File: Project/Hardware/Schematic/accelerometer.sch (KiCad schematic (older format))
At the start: 2 parts, among them U3 lis3dh_board

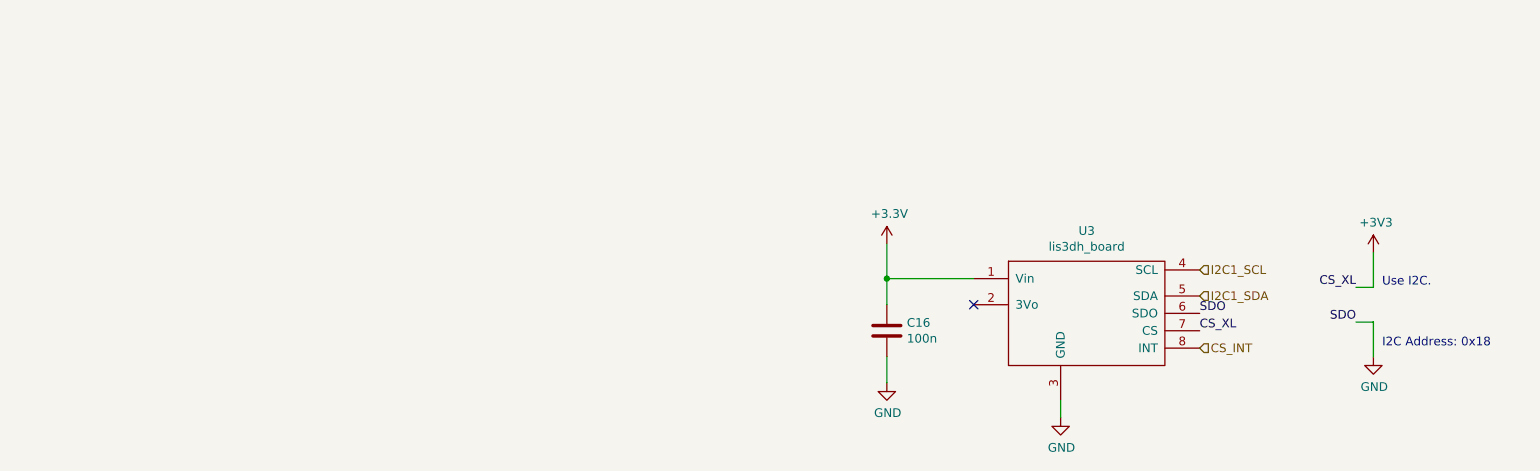
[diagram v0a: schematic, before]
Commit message: Intermediate...
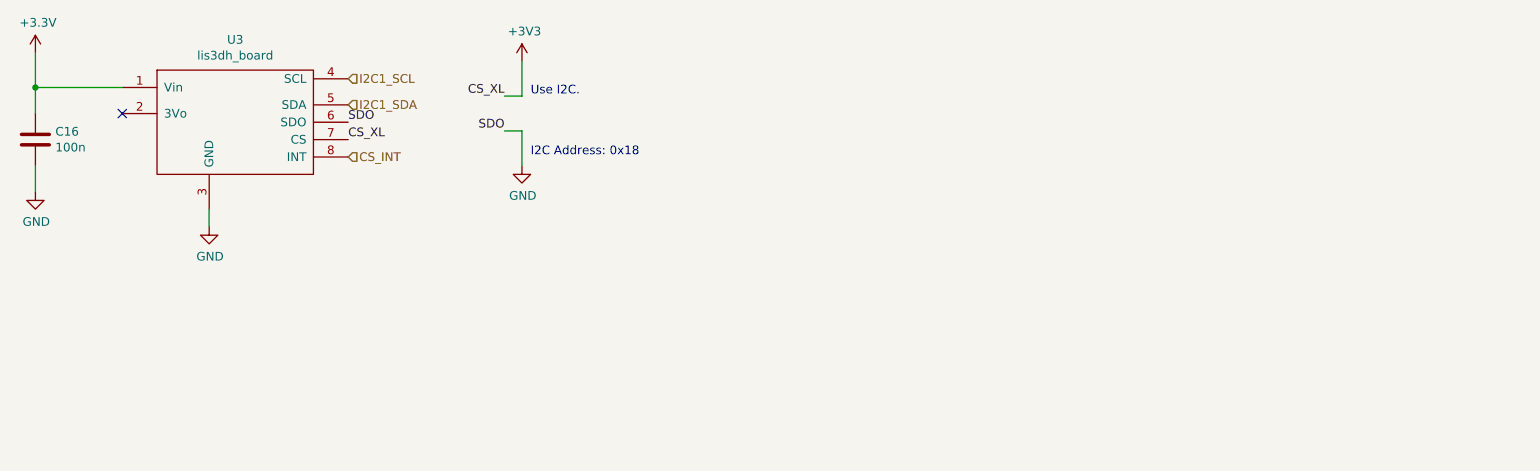
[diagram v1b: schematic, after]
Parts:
- C16: footprint (none) -> Capacitor_SMD:C_0805_2012Metric_Pad1.15x1.40mm_HandSolder
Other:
- moved on the sheet: C16, U3
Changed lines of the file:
@@
 EELAYER 26 0
 EELAYER END
-$Descr A4 11693 8268
+$Descr User 5512 5512
 encoding utf-8
 Sheet 2 7
 Title ""
-Date ""
-Rev ""
-Comp ""
+Date "2019-02-12"
+Rev "1"
+Comp "PASC"
 Comment1 ""
 Comment2 ""
@@
 L power:+3.3V #PWR0120
 U 1 1 5C5AB0A3
-P 6200 2950
-F 0 "#PWR0120" H 6200 2800 50  0001 C CNN
-F 1 "+3.3V" H 6215 3123 50  0000 C CNN
-F 2 "" H 6200 2950 50  0001 C CNN
-F 3 "" H 6200 2950 50  0001 C CNN
-	1    6200 2950
+P 1300 1850
+F 0 "#PWR0120" H 1300 1700 50  0001 C CNN
+F 1 "+3.3V" H 1315 2023 50  0000 C CNN
+F 2 "" H 1300 1850 50  0001 C CNN
+F 3 "" H 1300 1850 50  0001 C CNN
+	1    1300 1850
 	1    0    0    -1
 $EndComp
 Wire Wire Line
-	6200 2950 6200 3150
+	1300 1850 1300 2050
 Wire Wire Line
-	6700 3150 6200 3150
+	1800 2050 1300 2050
 $Comp
 L power:GND #PWR0121
 U 1 1 5C59F3FC
-P 7200 3950
-F 0 "#PWR0121" H 7200 3700 50  0001 C CNN
-F 1 "GND" H 7205 3777 50  0000 C CNN
-F 2 "" H 7200 3950 50  0001 C CNN
-F 3 "" H 7200 3950 50  0001 C CNN
-	1    7200 3950
+P 2300 2850
+F 0 "#PWR0121" H 2300 2600 50  0001 C CNN
+F 1 "GND" H 2305 2677 50  0000 C CNN
+F 2 "" H 2300 2850 50  0001 C CNN
+F 3 "" H 2300 2850 50  0001 C CNN
+	1    2300 2850
 	1    0    0    -1
 $EndComp
 Wire Wire Line
-	7200 3850 7200 3950
+	2300 2750 2300 2850
 $Comp
 L power:GND #PWR0122
 U 1 1 5C59F76F
-P 9000 3600
-F 0 "#PWR0122" H 9000 3350 50  0001 C CNN
-F 1 "GND" H 9005 3427 50  0000 C CNN
-F 2 "" H 9000 3600 50  0001 C CNN
-F 3 "" H 9000 3600 50  0001 C CNN
-	1    9000 3600
+P 4100 2500
+F 0 "#PWR0122" H 4100 2250 50  0001 C CNN
+F 1 "GND" H 4105 2327 50  0000 C CNN
+F 2 "" H 4100 2500 50  0001 C CNN
+F 3 "" H 4100 2500 50  0001 C CNN
+	1    4100 2500
 	1    0    0    -1
 $EndComp
-NoConn ~ 6700 3300
+NoConn ~ 1800 2200
 $Comp
 L Device:C C16
 U 1 1 5C5A61DB
-P 6200 3450
-F 0 "C16" H 6315 3496 50  0000 L CNN
-F 1 "100n" H 6315 3405 50  0000 L CNN
-F 2 "" H 6238 3300 50  0001 C CNN
-F 3 "~" H 6200 3450 50  0001 C CNN
-	1    6200 3450
+P 1300 2350
+F 0 "C16" H 1415 2396 50  0000 L CNN
+F 1 "100n" H 1415 2305 50  0000 L CNN
+F 2 "Capacitor_SMD:C_0805_2012Metric_Pad1.15x1.40mm_HandSolder" H 1338 2200 50  0001 C CNN
+F 3 "~" H 1300 2350 50  0001 C CNN
+	1    1300 2350
 	1    0    0    -1
 $EndComp
@@
 L power:GND #PWR0123
 U 1 1 5C5A62A1
-P 6200 3750
-F 0 "#PWR0123" H 6200 3500 50  0001 C CNN
-F 1 "GND" H 6205 3577 50  0000 C CNN
-F 2 "" H 6200 3750 50  0001 C CNN
-F 3 "" H 6200 3750 50  0001 C CNN
-	1    6200 3750
+P 1300 2650
+F 0 "#PWR0123" H 1300 2400 50  0001 C CNN
+F 1 "GND" H 1305 2477 50  0000 C CNN
+F 2 "" H 1300 2650 50  0001 C CNN
+F 3 "" H 1300 2650 50  0001 C CNN
+	1    1300 2650
 	1    0    0    -1
 $EndComp
 Wire Wire Line
-	6200 3150 6200 3300
-Connection ~ 6200 3150
+	1300 2050 1300 2200
+Connection ~ 1300 2050
 Wire Wire Line
-	6200 3600 6200 3750
-Text Notes 9050 3550 0    50   ~ 0
+	1300 2500 1300 2650
+Text Notes 4150 2450 0    50   ~ 0
 I2C Address: 0x18
-Text Label 8000 3350 0    50   ~ 0
+Text Label 3100 2250 0    50   ~ 0
 SDO
 Wire Wire Line
-	9000 3400 8900 3400
+	4100 2300 4000 2300
 Wire Wire Line
-	9000 3400 9000 3600
-Text Label 8900 3400 2    50   ~ 0
+	4100 2300 4100 2500
+Text Label 4000 2300 2    50   ~ 0
 SDO
-Text Label 8000 3450 0    50   ~ 0
+Text Label 3100 2350 0    50   ~ 0
 CS_XL
 $Comp
 L power:+3V3 #PWR0124
 U 1 1 5C5D1727
-P 9000 3000
-F 0 "#PWR0124" H 9000 2850 50  0001 C CNN
-F 1 "+3V3" H 9015 3173 50  0000 C CNN
-F 2 "" H 9000 3000 50  0001 C CNN
-F 3 "" H 9000 3000 50  0001 C CNN
-	1    9000 3000
+P 4100 1900
+F 0 "#PWR0124" H 4100 1750 50  0001 C CNN
+F 1 "+3V3" H 4115 2073 50  0000 C CNN
+F 2 "" H 4100 1900 50  0001 C CNN
+F 3 "" H 4100 1900 50  0001 C CNN
+	1    4100 1900
 	1    0    0    -1
 $EndComp
 Wire Wire Line
-	9000 3000 9000 3200
+	4100 1900 4100 2100
 Wire Wire Line
-	9000 3200 8900 3200
-Text Label 8900 3200 2    50   ~ 0
+	4100 2100 4000 2100
+Text Label 4000 2100 2    50   ~ 0
 CS_XL
-Text Notes 9050 3200 0    50   ~ 0
+Text Notes 4150 2100 0    50   ~ 0
 Use I2C.
-Text HLabel 8000 3100 2    50   Input ~ 0
+Text HLabel 3100 2000 2    50   Input ~ 0
 I2C1_SCL
-Text HLabel 8000 3250 2    50   Input ~ 0
+Text HLabel 3100 2150 2    50   Input ~ 0
 I2C1_SDA
-Text HLabel 8000 3550 2    50   Input ~ 0
+Text HLabel 3100 2450 2    50   Input ~ 0
 CS_INT
 $Comp
 L PASC:lis3dh_board U3
 U 1 1 5C5E039C
-P 7350 3350
-F 0 "U3" H 7350 3825 50  0000 C CNN
-F 1 "lis3dh_board" H 7350 3734 50  0000 C CNN
-F 2 "PASC:LIS3DH" H 7350 3350 50  0001 C CNN
-F 3 "" H 7350 3350 50  0001 C CNN
-	1    7350 3350
+P 2450 2250
+F 0 "U3" H 2450 2725 50  0000 C CNN
+F 1 "lis3dh_board" H 2450 2634 50  0000 C CNN
+F 2 "PASC:LIS3DH" H 2450 2250 50  0001 C CNN
+F 3 "" H 2450 2250 50  0001 C CNN
+	1    2450 2250
 	1    0    0    -1
 $EndComp
